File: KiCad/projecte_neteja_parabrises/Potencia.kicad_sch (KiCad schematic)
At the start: 1 part, among them J2 Conn_01x09_Pin

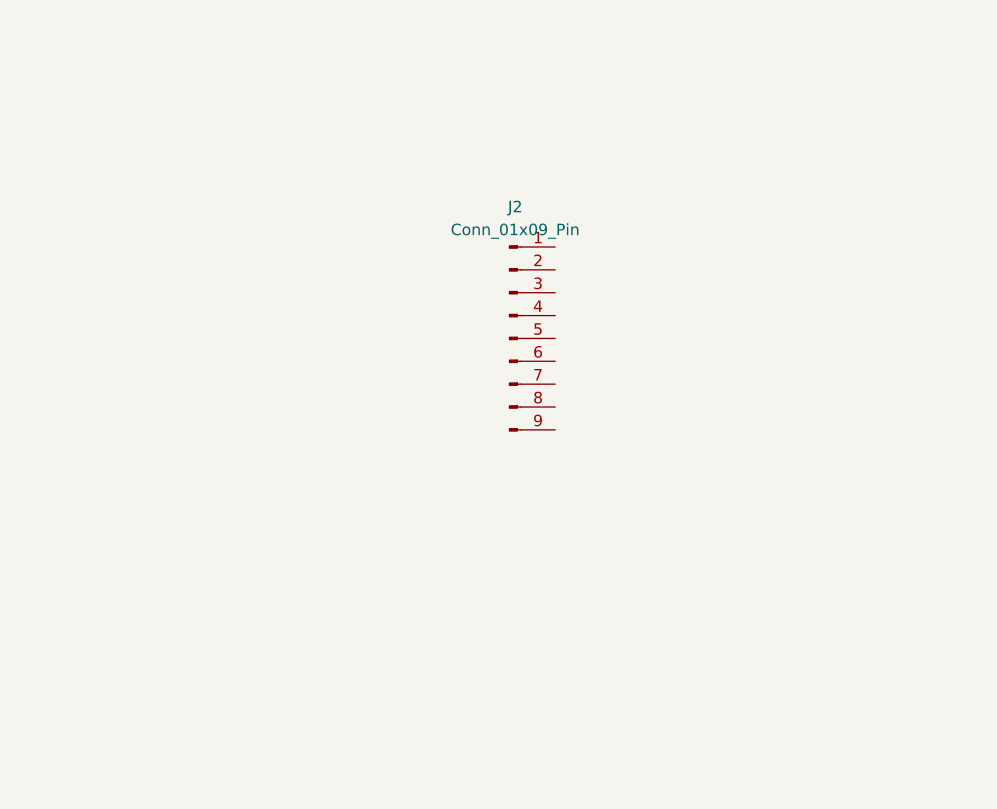
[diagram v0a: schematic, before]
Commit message: Potencia actualizada
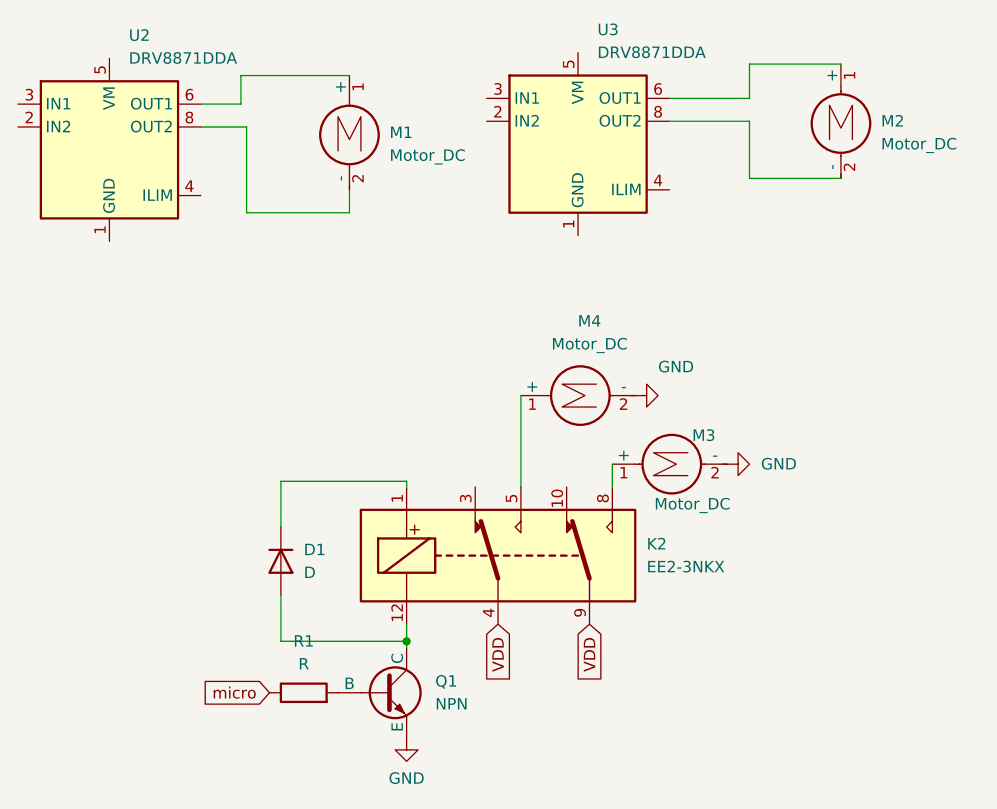
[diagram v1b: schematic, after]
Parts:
- removed J2: Conn_01x09_Pin, symbol Connector:Conn_01x09_Pin
- added D1: D, symbol Device:D
- added K2: EE2-3NKX, Relay_SMD:Relay_DPDT_Kemet_EE2_NUX_NKX, symbol Relay:EE2-3NKX
- added M1, M2, M3, M4: Motor_DC, symbol Motor:Motor_DC
- added Q1: NPN, symbol Simulation_SPICE:NPN
- added R1: R, symbol Device:R
- added U2, U3: DRV8871DDA, Package_SO:Texas_HTSOP-8-1EP_3.9x4.9mm_P1.27mm_EP2.95x4.9mm_Mask2.4x3.1mm_ThermalVias, symbol Driver_Motor:DRV8871DDA
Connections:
- new net: D1.1 (K), K2.1
- new net: D1.2 (A), K2.12, Q1.1 (C)
- new net: U2.1 (GND), U2.7 (GND), U2.9 (GND)
- new net: M1.1 (+), U2.6 (OUT1)
- new net: M1.2 (-), U2.8 (OUT2)
- new net: Q1.2 (B), R1.2
- new net: U3.1 (GND), U3.7 (GND), U3.9 (GND)
- new net: M2.1 (+), U3.6 (OUT1)
- new net: M2.2 (-), U3.8 (OUT2)
- new net: K2.8, M3.1 (+)
- new net: K2.5, M4.1 (+)
- new net GND: M3.2 (-), M4.2 (-), Q1.3 (E)
- new net VDD: K2.4, K2.9
- new net micro: R1.1
